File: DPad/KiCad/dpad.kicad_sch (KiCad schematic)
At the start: 17 parts, among them SW1 SW_Push, SW2 SW_Push, SW3 SW_Push, SW4 SW_Push

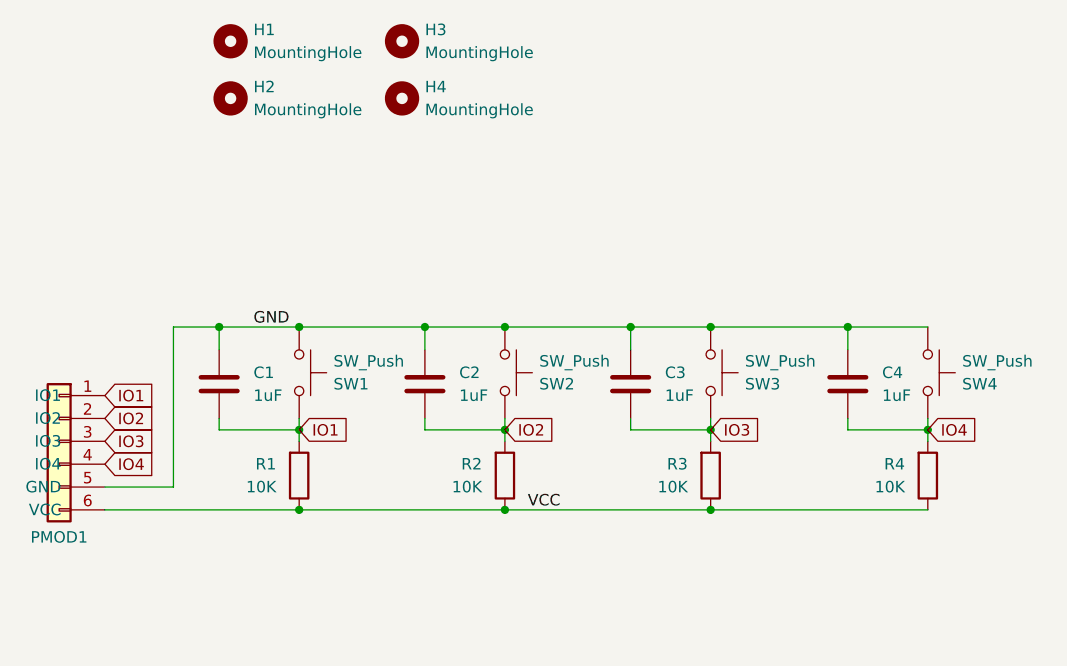
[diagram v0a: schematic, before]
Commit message: Deployed d972a79 with MkDocs version: 1.6.0
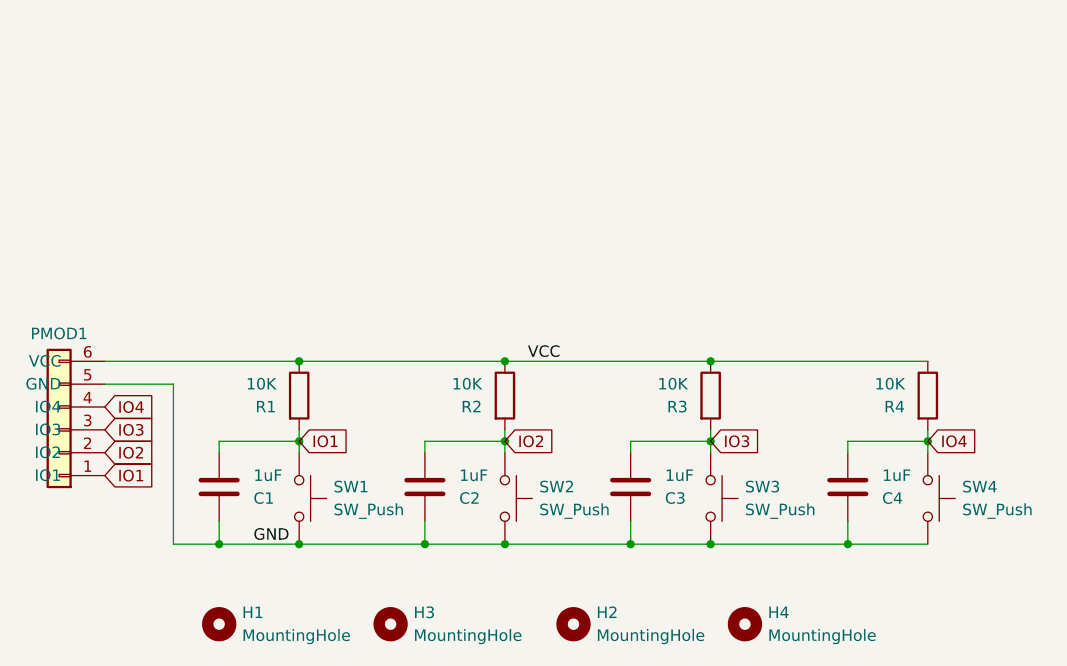
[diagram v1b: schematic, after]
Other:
- moved on the sheet: C1, C2, C3, C4, H1, H2, H3, H4, PMOD1, R1, R2, R3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
